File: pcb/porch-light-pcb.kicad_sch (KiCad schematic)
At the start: 2 parts

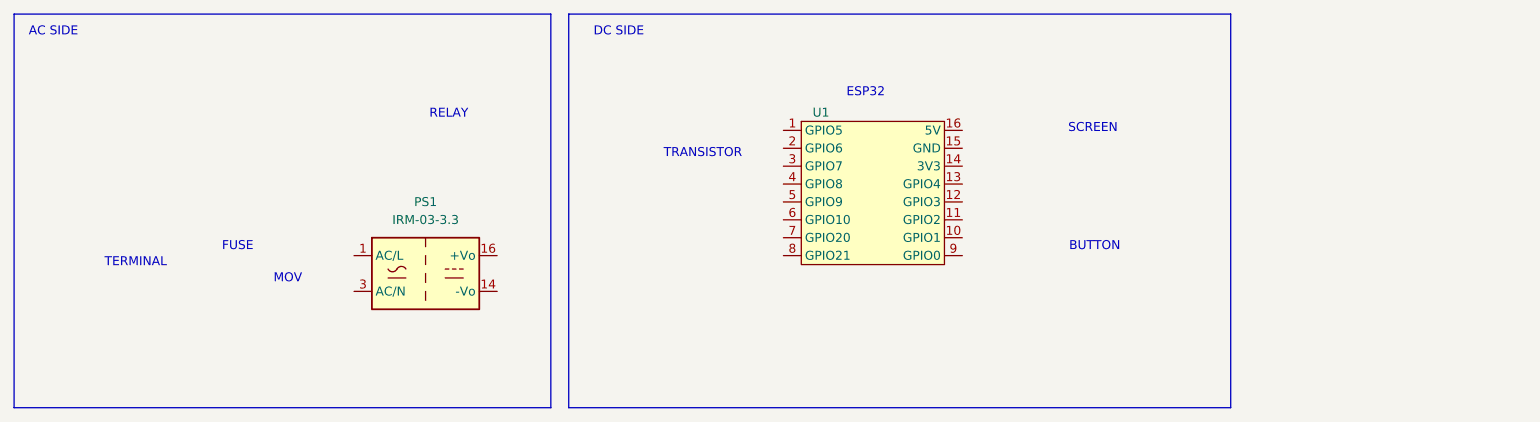
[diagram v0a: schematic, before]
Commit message: preliminary circuit design
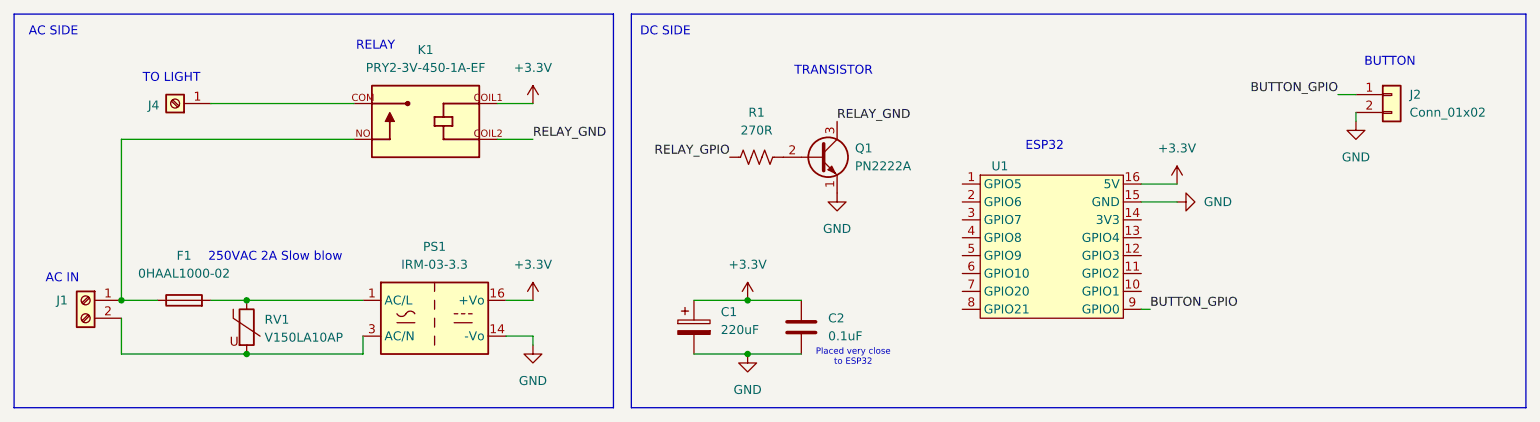
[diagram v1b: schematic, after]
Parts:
- added C1: 220uF, Capacitor_THT:CP_Radial_D5.0mm_P2.50mm, symbol Device:C_Polarized
- added C2: 0.1uF, Capacitor_SMD:C_0603_1608Metric_Pad1.08x0.95mm_HandSolder, symbol Device:C
- added F1: 0HAAL1000-02, symbol Device:Fuse
- added J1: Screw_Terminal_01x02, symbol Connector:Screw_Terminal_01x02
- added J2: Conn_01x02, Connector_PinHeader_2.54mm:PinHeader_1x02_P2.54mm_Vertical, symbol Connector_Generic:Conn_01x02
- added J4: Screw_Terminal_01x01, symbol Connector:Screw_Terminal_01x01
- added K1: PRY2-3V-450-1A-EF, PRY2_3V_450_1A_EF:RELAY_PRY2-3V-450-1A-EF, symbol PRY2-3V-450-1A-EF:PRY2-3V-450-1A-EF
- added Q1: PN2222A, Package_TO_SOT_THT:TO-92_Inline, symbol Transistor_BJT:PN2222A
- added R1: 270R, symbol Device:R_US
- added RV1: V150LA10AP, symbol Device:Varistor
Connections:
- net GND: now reaches U1.15 (GND)
- net GND: now also PS1.14 (-Vo), C1.2, C2.2, J2.2 (Pin_2), Q1.1 (E)
- net +3.3V: now reaches U1.16 (5V)
- net +3.3V: now also PS1.16 (+Vo), C1.1, C2.1, K1.COIL1
- net BUTTON_GPIO: now reaches U1.9 (GPIO0)
- net BUTTON_GPIO: now also J2.1 (Pin_1)
- net at PS1.1 (AC/L): now also F1.2, RV1.1
- net at PS1.3 (AC/N): now also J1.2 (Pin_2), RV1.2
- new net: F1.1, J1.1 (Pin_1), K1.NO
- new net: Q1.2 (B), R1.2
- new net: J4.1 (Pin_1), K1.COM
- new net RELAY_GND: K1.COIL2, Q1.3 (C)
- new net RELAY_GPIO: R1.1
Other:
- note added: "250VAC 2A Slow blow"
- note added: "AC IN"
- note added: "Placed very close to ESP32"
- note added: "TO LIGHT"
- note removed: "FUSE"
- note removed: "MOV"
- note removed: "SCREEN"
- note removed: "TERMINAL"
- moved on the sheet: PS1, U1
